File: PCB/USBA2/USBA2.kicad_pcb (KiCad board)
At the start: 2 copper layers, 15.9 x 13.8 mm, 19 parts, among them J1 USB_A, J2 Shelly, U1 ESP32-PICO-MINI-02, U2 LMR16006YDDCR, U4 QR

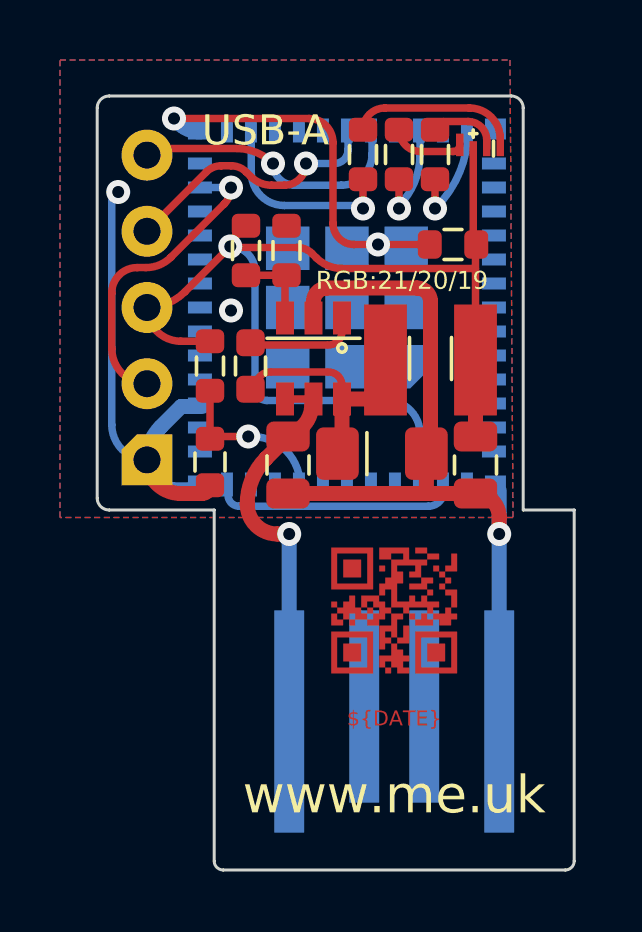
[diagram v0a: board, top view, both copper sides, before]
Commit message: New layoput
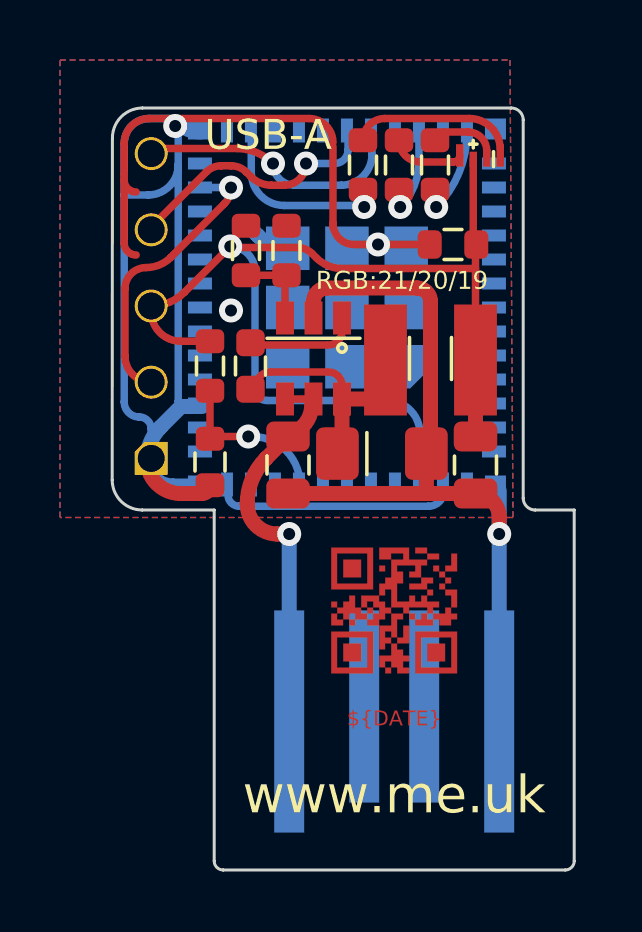
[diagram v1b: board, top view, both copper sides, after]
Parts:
- moved D1 0.35 mm to (124.4, 107.3)
- moved R1 0.35 mm to (122.9, 107.5)
- moved R2 0.35 mm to (120.5, 107.5)
- moved R3 0.35 mm to (121.7, 107.5)
- moved J2 0.15 mm to (113.4, 112.2)
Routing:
- net GND: track 47.4 -> 71.6 mm, vias 5 -> 4
- net GPIO0: track 10.3 -> 9.70 mm
- net +3.3V: track 35.5 -> 34.9 mm
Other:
- board size 15.9 x 13.8 mm -> 15.4 x 13.4 mm
